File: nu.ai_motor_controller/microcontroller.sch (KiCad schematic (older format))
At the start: 35 parts, among them J10 Conn_02x05_Odd_Even, J11 DX4R105JJCR1800, J9 Conn_02x12_Odd_Even, SW1 TACTILE_SWITCH, U9 ATmega32U4-AU, Y1 7M-16.000MAAE-T

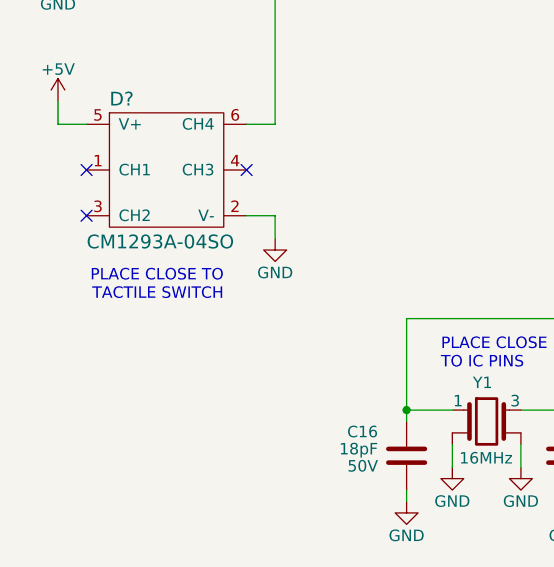
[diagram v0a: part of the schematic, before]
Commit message: automated commit
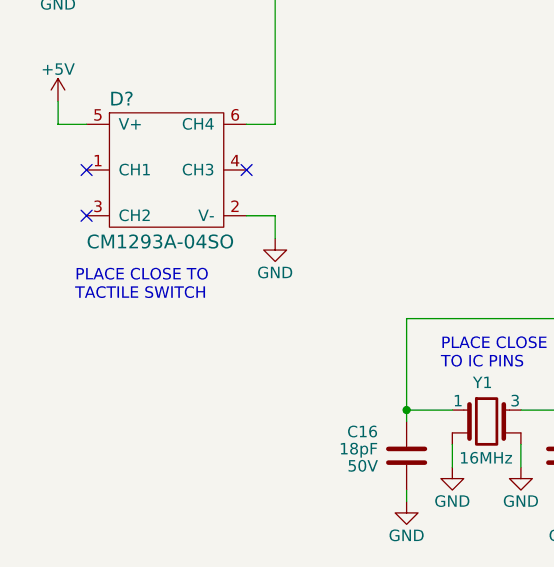
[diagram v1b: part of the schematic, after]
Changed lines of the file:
@@
 	1725 1800 1600 1800
 Connection ~ 1725 950
-Text Notes 1500 2575 2    50   ~ 0
+Text Notes 850  2575 0    50   ~ 0
 PLACE CLOSE TO\nTACTILE SWITCH
 $Comp
